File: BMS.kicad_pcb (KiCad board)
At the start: 6 copper layers, 67 x 60 mm, 170 parts, among them J1 UJ20-C-H-G-SMT-1-P16-TR, J10 Conn_01x02_Pin, J11 Conn_01x02_Pin, J12 Conn_01x02_Pin, J13 Conn_01x02_Pin, J2 Conn_01x02_Socket, J4 Conn_01x04_Socket, J5 Conn_01x03_Socket, J6 Conn_01x03_Socket, J7 Conn_01x03_Socket, J8 Conn_01x10_Pin, J9 Conn_01x02_Pin, Q1 FZT853TA, Q2 PSMN3R7-100BSE, Q3 PSMN3R7-100BSE, Q4 PSMN3R7-100BSE, Q5 PSMN3R7-100BSE, U1 USBLC6-2SC6, U10 SQ1464EEH-T1_GE3, U11 MP2790DFP-0000-T, U2 USBLC6-2SC6, U3 RP2350A, U4 TPS7B8133QDGNRQ1, U5 SQ1464EEH-T1_GE3, U6 SQ1464EEH-T1_GE3, U7 SQ1464EEH-T1_GE3, U8 SQ1464EEH-T1_GE3, U9 SQ1464EEH-T1_GE3, X1 ABM8-272-T3

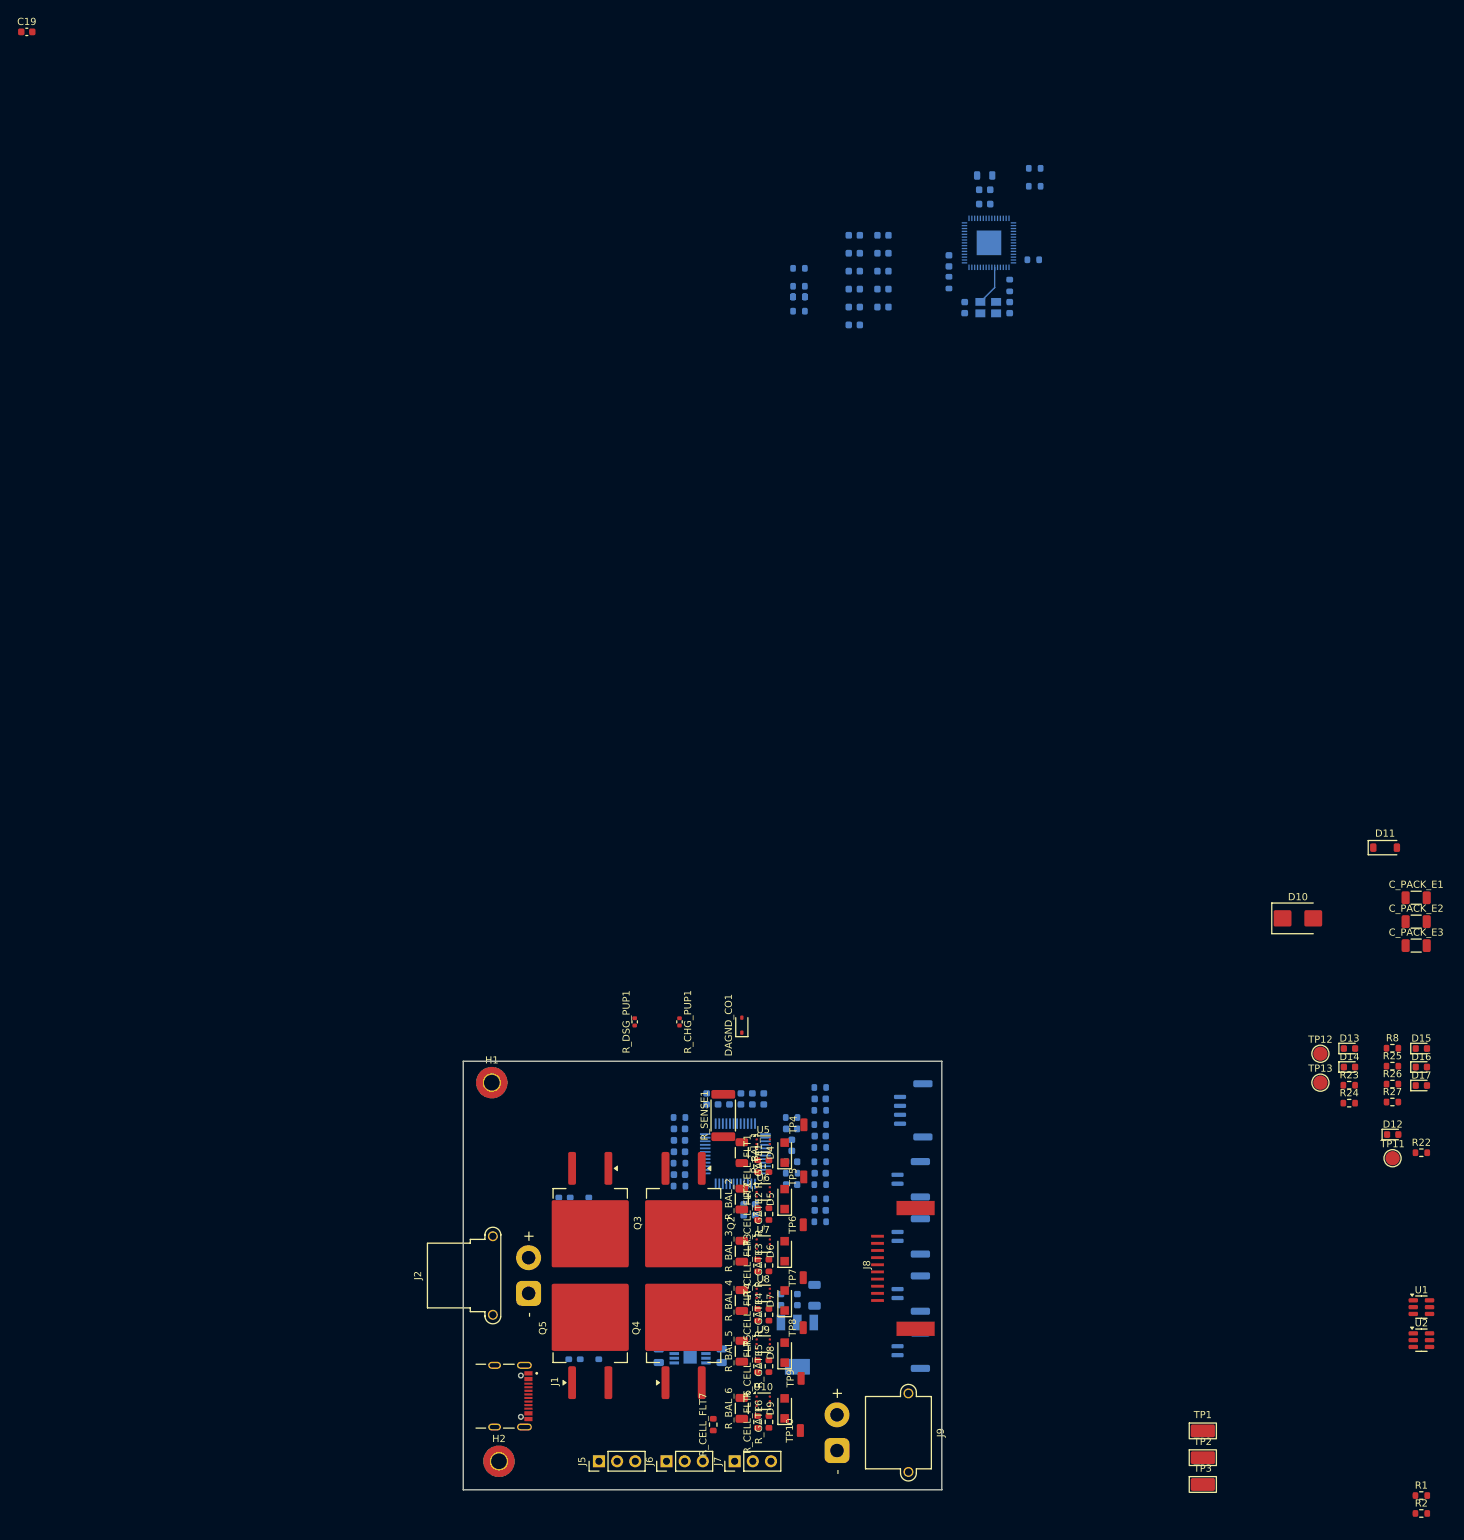
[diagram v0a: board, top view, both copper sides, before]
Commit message: Prelim placement done
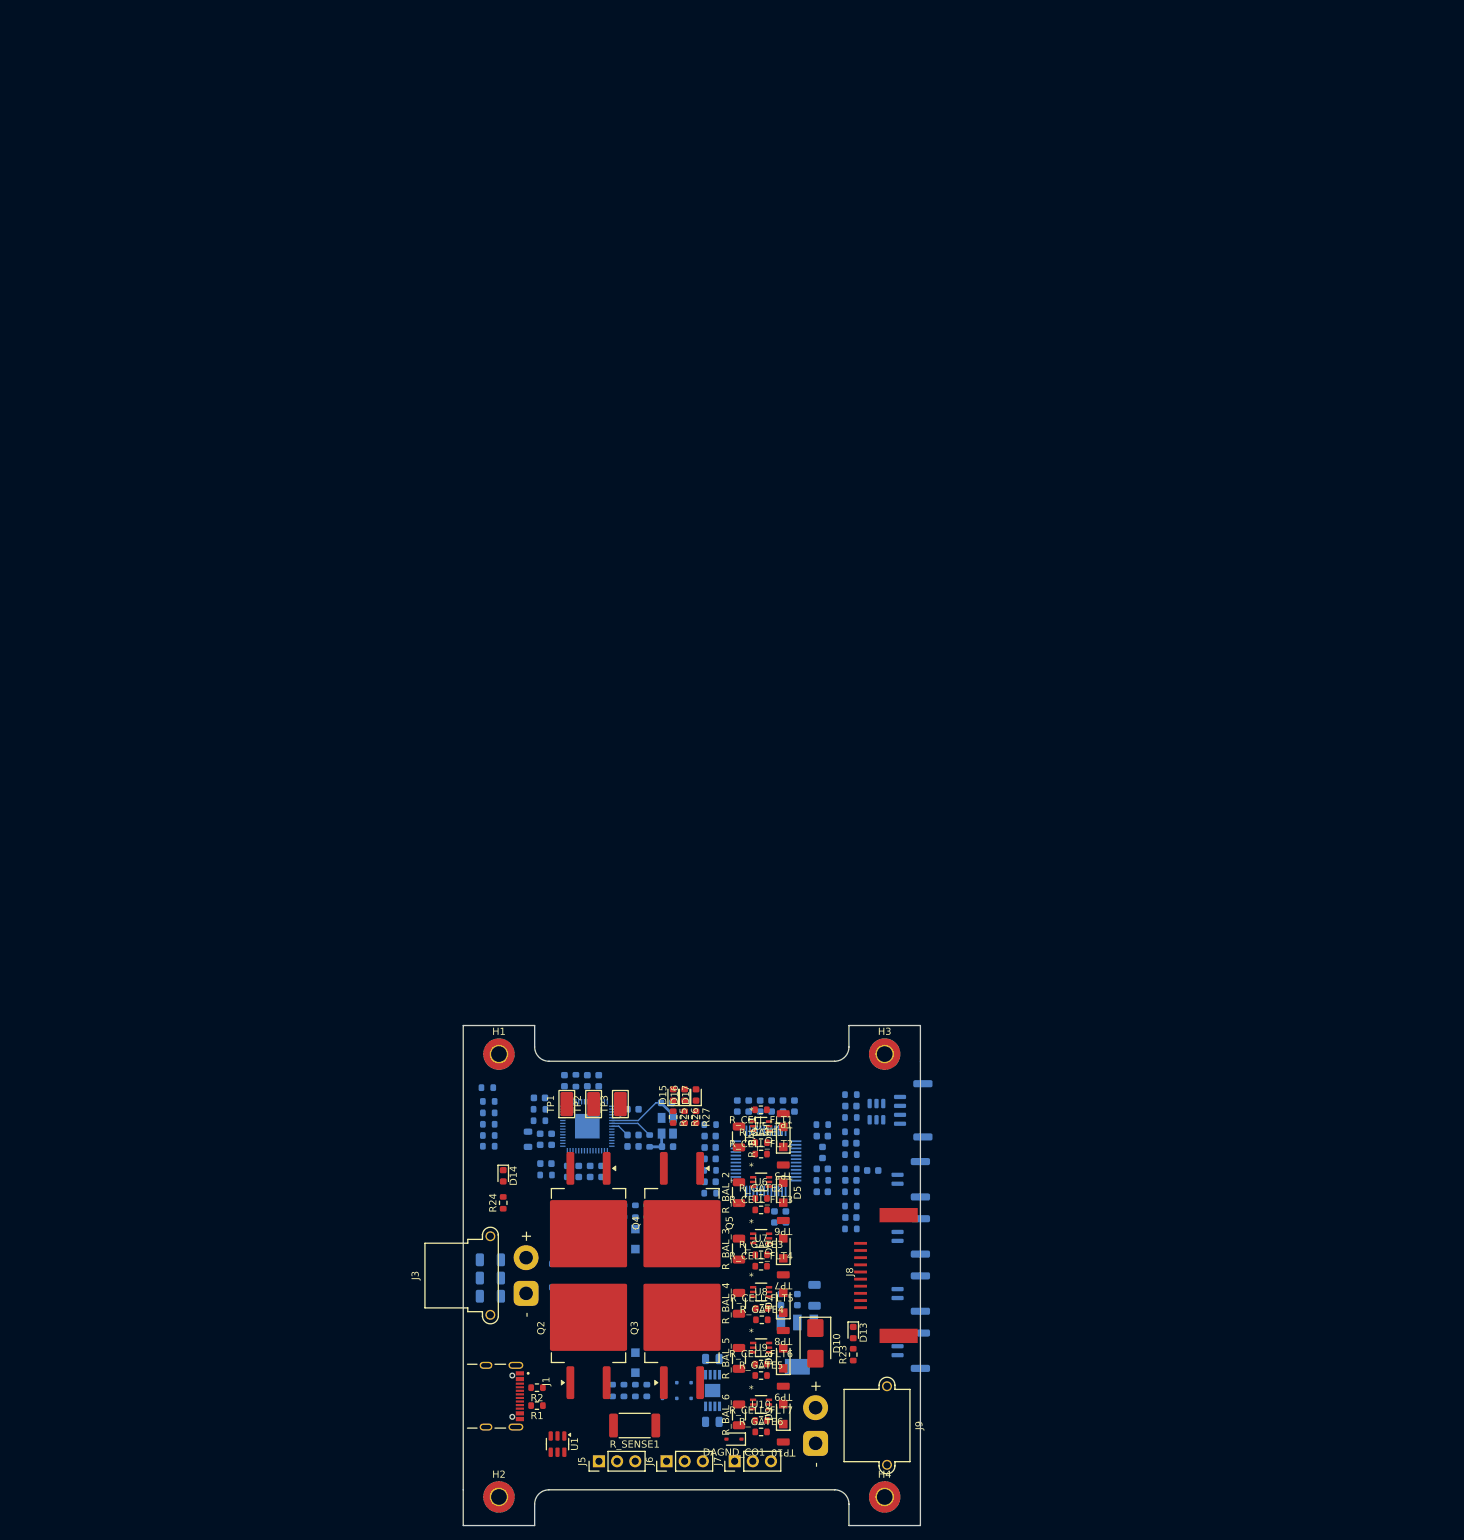
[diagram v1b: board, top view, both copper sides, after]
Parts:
- removed D12: LED, LED_SMD:LED_0603_1608Metric
- removed J2: Conn_01x02_Socket, Connector_AMASS:AMASS_XT30PW-F_1x02_P2.50mm_Horizontal
- removed R22: R, Resistor_SMD:R_0603_1608Metric
- removed TP11, TP12, TP13: TestPoint, TestPoint:TestPoint_Pad_D2.0mm
- added H3: MountingHole, MountingHole:MountingHole_2.2mm_M2_Pad_TopBottom, F.Cu at (169.0, 59.0)
- added H4: MountingHole, MountingHole:MountingHole_2.2mm_M2_Pad_TopBottom, F.Cu at (169.0, 121.0)
- added J3: Conn_01x02_Socket, Connector_AMASS:AMASS_XT30PW-F_1x02_P2.50mm_Horizontal, F.Cu at (118.8, 92.5)
- C19, C_PACK_E1, C_PACK_E2, C_PACK_E3, D11, R8, U2: moved to B.Cu
- R_CHG_PUP1, R_DSG_PUP1: footprint Resistor_SMD:R_0402_1005Metric -> Resistor_SMD:R_0603_1608Metric; moved to B.Cu
- U10, U5, U6, U7, U8, U9: footprint _BMS:SC70-6 -> _BMS:SC_4EEH-T1_GE3_VIS
- moved C19 198.6 mm to (167.3, 75.3)
- moved L1 149.3 mm to (119.1, 70.9), turned to 90 degrees
- moved R12 148.9 mm to (120.7, 66.7)
- moved R11 148.1 mm to (120.7, 68.3), turned to 180 degrees
- moved C15 146.8 mm to (120.8, 70.9), turned to 90 degrees
- moved C16 144.3 mm to (122.4, 70.9), turned to -90 degrees
- moved C_PACK_E1 141.1 mm to (113.8, 92.9)
- moved C_PACK_E2 138.9 mm to (113.8, 90.3)
- moved C14 138.4 mm to (121.6, 74.3), turned to 180 degrees
- moved C13 138.3 mm to (124.6, 75.4), turned to 90 degrees
- moved R13 137.1 mm to (121.6, 75.9), turned to 0 degrees
- moved C_PACK_E3 136.9 mm to (113.8, 87.8)
- moved U3 135.9 mm to (127.4, 69.1), turned to -90 degrees
- moved C12 135.4 mm to (126.2, 75.4), turned to -90 degrees
- moved C11 132.0 mm to (129.4, 75.4), turned to 90 degrees
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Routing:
- net /main/microcontroller/XOUT: track 0.00 -> 5.98 mm
- net /main/microcontroller/XIN: track 5.67 -> 10.7 mm
- net /main/microcontroller/XR: track 0.00 -> 3.59 mm
- net +1V1: track 0.00 -> 2.71 mm
- net +3V3: track 0.00 -> 2.68 mm
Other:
- board size 67 x 60 mm -> 64 x 70 mm
